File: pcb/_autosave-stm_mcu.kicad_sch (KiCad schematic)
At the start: 44 parts, among them J3 Micro_SD_Card, J7 Conn_ST_STDC14, U15 TXS02612RTW, U3 STM32H7S7L8H6H, U5 APS256XXN-OBR-BG, Y3 32.768kHz, Y4 40MHz(10ppm)

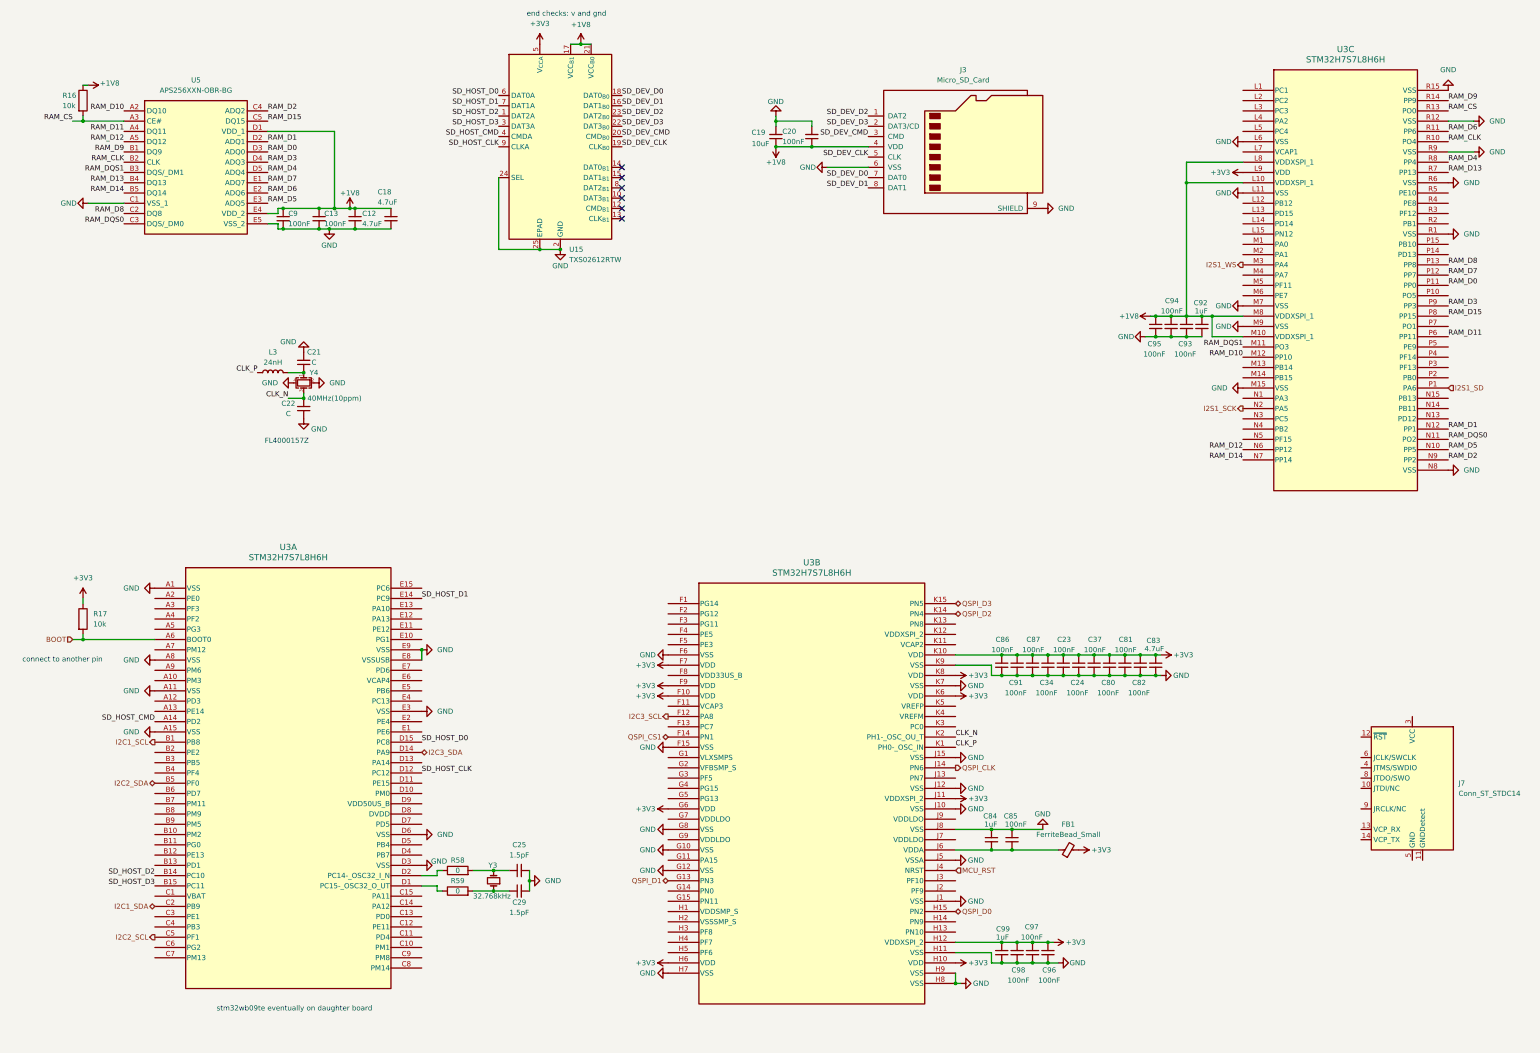
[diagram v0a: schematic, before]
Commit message: returning and reorganizing
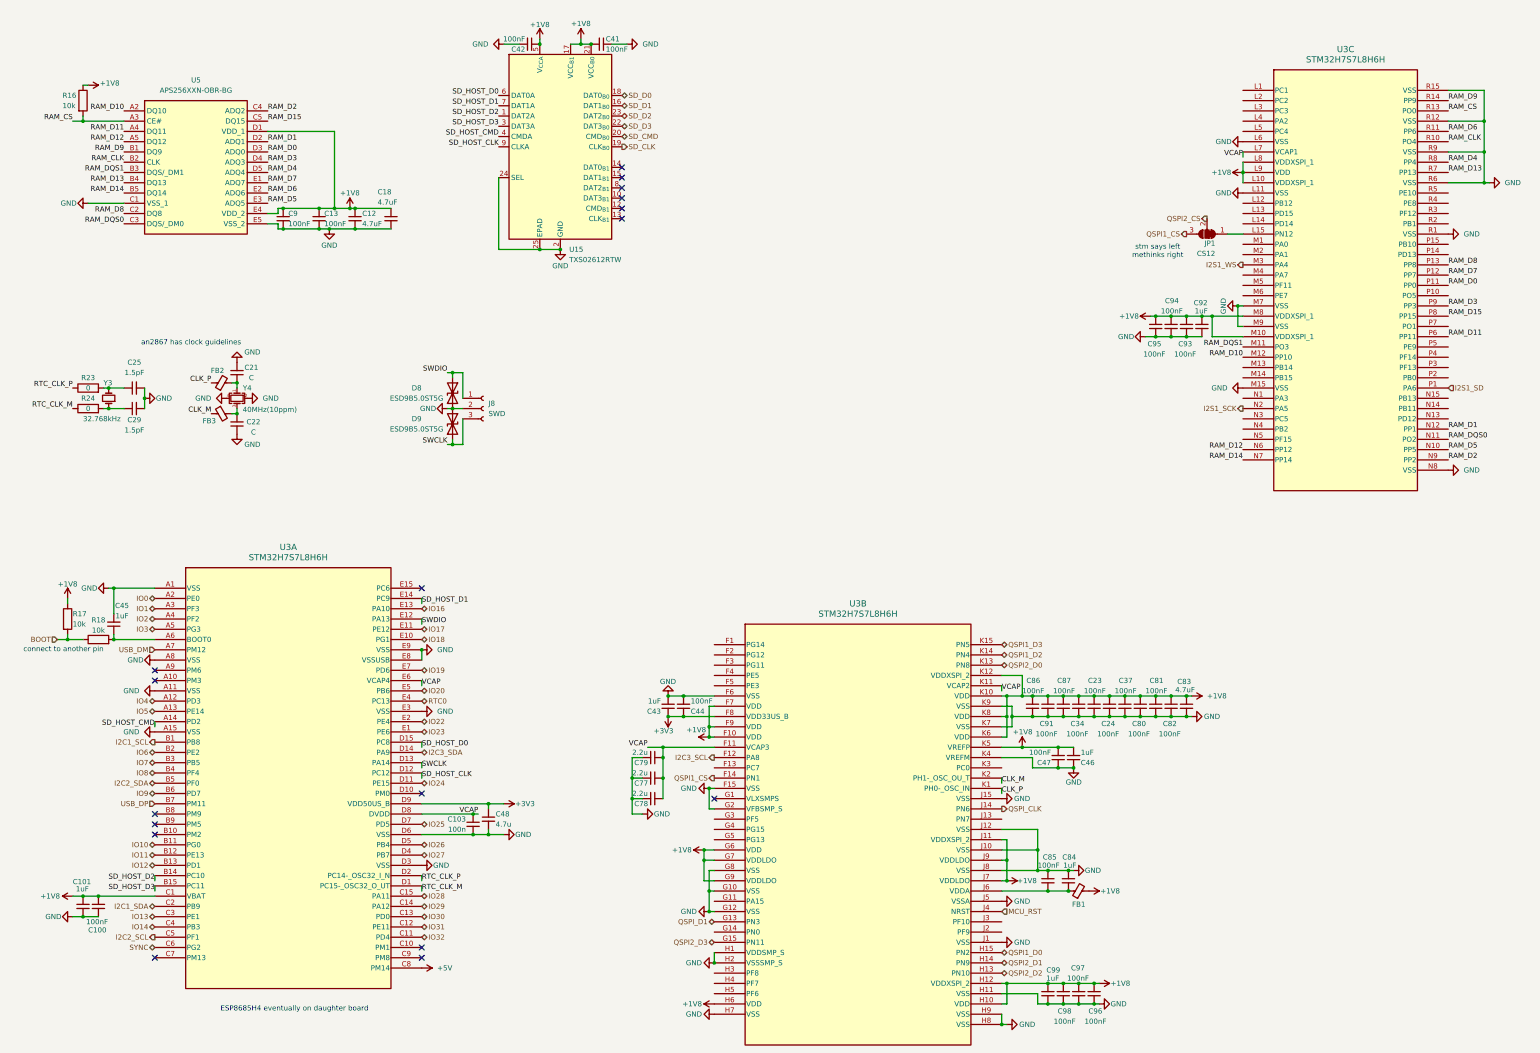
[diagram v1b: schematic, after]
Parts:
- removed C19: 10uF, symbol Device:C_Small
- removed C20: 100nF, symbol Device:C_Small
- removed J3: Micro_SD_Card, Connector_Card:microSD_HC_Molex_104031-0811, symbol Connector:Micro_SD_Card
- removed J7: Conn_ST_STDC14, Connector_PinHeader_1.27mm:PinHeader_2x07_P1.27mm_Vertical_SMD, symbol Connector:Conn_ST_STDC14
- removed L3: 24nH, Inductor_SMD:L_Coilcraft_XFL2010, symbol Device:L
- removed R58, R59: 0, symbol Device:R
- added C100, C41, C42, C44, C47: 100nF, symbol Device:C_Small
- added C101, C43, C46: 1uF, symbol Device:C_Small
- added C103: 100n, symbol Device:C_Small
- added C45: 1uF, Capacitor_SMD:C_0402_1005Metric, symbol Device:C_Small
- added C48: 4.7u, symbol Device:C_Small
- added C77, C78, C79: 2.2u, symbol Device:C_Small
- added D8, D9: ESD9B5.0ST5G, Diode_SMD:D_SOD-923, symbol Diode:ESD9B5.0ST5G
- added FB2, FB3: ~, symbol Device:FerriteBead_Small
- added J8: SWD, symbol Connector:Conn_01x03_Socket
- added JP1: CS12, Jumper:SolderJumper-3_P1.3mm_Open_RoundedPad1.0x1.5mm_NumberLabels, symbol Jumper:SolderJumper_3_Bridged12
- added R18: 10k, symbol Device:R
- added R23, R24: 0, symbol Device:R
- FB1: value FerriteBead_Small -> ~
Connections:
- net +1V8: now also C23.1, C24.1, C34.1, C37.1, C80.1, C81.1, C82.1, C83.1, C86.1, C87.1, C91.1, C96.1, C97.1, C98.1, C99.1, FB1.2, R17.1, U15.5 (V_{CCA}), U3.C1 (VBAT), U3.F10 (VDD), U3.F7 (VDD), U3.F9 (VDD), U3.G6 (VDD), U3.G7 (VDDLDO), U3.G9 (VDDLDO), U3.H10 (VDD), U3.H12 (VDDXSPI_2), U3.H6 (VDD), U3.J11 (VDDXSPI_2), U3.J7 (VDDLDO), U3.J9 (VDDLDO), U3.K10 (VDD), U3.K12 (VDDXSPI_2), U3.K5 (VREFP), U3.K6 (VDD), U3.K8 (VDD), U3.L9 (VDD), C100.2, C101.2, C41.2, C42.1, C46.2, C47.2
- net +3V3: now also U3.D9 (VDD50US_B), U3.F8 (VDD33US_B), C43.1, C44.1, C48.1; no longer C23.1, C24.1, C34.1, C37.1, C80.1, C81.1, C82.1, C83.1, C86.1, C87.1, C91.1, C96.1, C97.1, C98.1, C99.1, FB1.2, R17.1, U15.5 (V_{CCA}), U3.F10 (VDD), U3.F7 (VDD), U3.F9 (VDD), U3.G6 (VDD), U3.H10 (VDD), U3.H12 (VDDXSPI_2), U3.H6 (VDD), U3.J11 (VDDXSPI_2), U3.K10 (VDD), U3.K6 (VDD), U3.K8 (VDD), U3.L9 (VDD)
- net BOOT: now also R18.1; no longer U3.A6 (BOOT0)
- net CLK_P: now also FB2.1
- net GND: now also U3.G2 (VFBSMP_S), U3.H1 (VDDSMP_S), U3.H2 (VSSSMP_S), U3.K4 (VREFM), C100.1, C101.1, C103.2, C41.1, C42.2, C43.2, C44.2, C45.2, C46.1, C47.1, C48.2, C77.2, C78.2, C79.2, D8.1 (A1), D9.2 (A2), J8.2 (Pin_2)
- net VCAP: now reaches U3.F11 (VCAP3)
- net VCAP: now also U3.D8 (DVDD), U3.E6 (VCAP4), U3.K11 (VCAP2), U3.L7 (VCAP1), C103.1, C77.1, C78.1, C79.1
- net QSPI2_D3: now reaches U3.G15 (PN11)
- net QSPI2_D2: now reaches U3.H13 (PN10)
- net QSPI2_D1: now reaches U3.H14 (PN9)
- net QSPI2_D0: now reaches U3.K13 (PN8)
- net RTC_CLK_P: now reaches U3.D2 (PC14-_OSC32_I_N)
- net RTC_CLK_P: now also R23.1
- net at C25.1, Y3.2: now also R23.2
- net at U3.L15 (PN12): now also JP1.1 (A)
- net IO4: now reaches U3.A12 (PD3)
- net IO5: now reaches U3.A13 (PE14)
- net IO0: now reaches U3.A2 (PE0)
- net IO1: now reaches U3.A3 (PF3)
- net IO2: now reaches U3.A4 (PF2)
- net IO3: now reaches U3.A5 (PG3)
- net USB_DM: now reaches U3.A7 (PM12)
- net IO10: now reaches U3.B11 (PG0)
- net IO11: now reaches U3.B12 (PE13)
- net IO12: now reaches U3.B13 (PD1)
- net IO6: now reaches U3.B2 (PE2)
- net IO7: now reaches U3.B3 (PB5)
- net IO8: now reaches U3.B4 (PF4)
- net IO9: now reaches U3.B6 (PD7)
- net USB_DP: now reaches U3.B7 (PM11)
- net IO32: now reaches U3.C11 (PD4)
- net IO31: now reaches U3.C12 (PE11)
- net IO30: now reaches U3.C13 (PD0)
- net IO29: now reaches U3.C14 (PA12)
- net IO28: now reaches U3.C15 (PA11)
- net IO13: now reaches U3.C3 (PE1)
- net IO14: now reaches U3.C4 (PB3)
- net SYNC: now reaches U3.C6 (PG2)
- net +5V: now reaches U3.C8 (PM14)
- net RTC_CLK_M: now reaches U3.D1 (PC15-_OSC32_O_UT)
- net RTC_CLK_M: now also R24.1
- net IO24: now reaches U3.D11 (PE15)
- net SWCLK: now reaches U3.D13 (PA14)
- net SWCLK: now also D9.1 (A1), J8.3 (Pin_3)
- net IO27: now reaches U3.D4 (PB7)
- net IO26: now reaches U3.D5 (PB4)
- net IO25: now reaches U3.D7 (PD5)
- net IO23: now reaches U3.E1 (PE6)
- net IO18: now reaches U3.E10 (PG1)
- net IO17: now reaches U3.E11 (PE12)
- net SWDIO: now reaches U3.E12 (PA13)
- net SWDIO: now also D8.2 (A2), J8.1 (Pin_1)
- net IO16: now reaches U3.E13 (PA10)
- net IO22: now reaches U3.E2 (PE4)
- net RTC0: now reaches U3.E4 (PC13)
- net IO20: now reaches U3.E5 (PB6)
- net IO19: now reaches U3.E7 (PD6)
- net at C21.1, Y4.1: now also FB2.2
- net at C29.1, Y3.1: now also R24.2
- net CLK_N: no longer names the net of C22.2, Y4.3
- net CLK_N: now also FB3.2; no longer U3.K2 (PH1-_OSC_OU_T)
- net QSPI_CS1 renamed QSPI1_CS
- net QSPI1_CS: now also JP1.3 (B)
- net QSPI_D0 renamed QSPI1_D0
- net QSPI_D2 renamed QSPI1_D2
- net QSPI_D3 renamed QSPI1_D3
- net SD_DEV_CLK renamed SD_CLK
- net SD_DEV_CMD renamed SD_CMD
- net SD_DEV_D0 renamed SD_D0
- net SD_DEV_D1 renamed SD_D1
- net SD_DEV_D2 renamed SD_D2
- net SD_DEV_D3 renamed SD_D3
- new net: C45.1, R18.2, U3.A6 (BOOT0)
- new net CLK_M: FB3.1, U3.K2 (PH1-_OSC_OU_T)
- new net QSPI2_CS: JP1.2 (C)
- no-connect marks 6 -> 17
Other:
- note added: "ESP8685H4 eventually on daughter board"
- note added: "an2867 has clock guidelines"
- note added: "stm says left methinks right"
- note removed: "FL4000157Z"
- note removed: "end checks: v and gnd"
- note removed: "stm32wb09te eventually on daughter board"
- moved on the sheet: C21, C22, C23, C24, C34, C37, C80, C81, C82, C83, C84, C86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
